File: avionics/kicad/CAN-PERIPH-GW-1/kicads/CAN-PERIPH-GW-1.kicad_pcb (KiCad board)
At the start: 2 copper layers, 49 x 25.5 mm, 32 parts, among them U1_1 MSPM0G3507, U2_1 SLB9670, U3_1 ISOW1044BDFMR, U4_1 ISOW1412

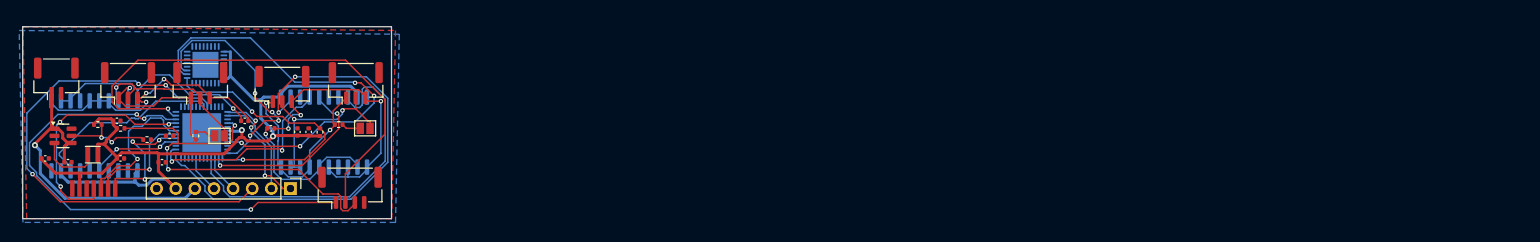
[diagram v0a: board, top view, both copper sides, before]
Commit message: just making everything shiny
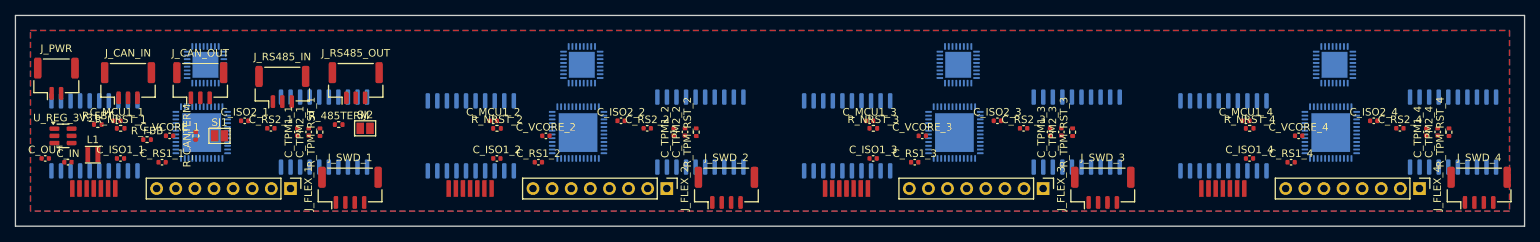
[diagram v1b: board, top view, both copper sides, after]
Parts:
- added C_ISO1_2: 100nF, Capacitor_SMD:C_0402_1005Metric, F.Cu at (194.0, 110.0)
- added C_ISO1_3: 100nF, Capacitor_SMD:C_0402_1005Metric, F.Cu at (244.0, 110.0)
- added C_ISO1_4: 100nF, Capacitor_SMD:C_0402_1005Metric, F.Cu at (294.0, 110.0)
- added C_ISO2_2: 1uF, Capacitor_SMD:C_0402_1005Metric, F.Cu at (210.5, 105.0)
- added C_ISO2_3: 1uF, Capacitor_SMD:C_0402_1005Metric, F.Cu at (260.5, 105.0)
- added C_ISO2_4: 1uF, Capacitor_SMD:C_0402_1005Metric, F.Cu at (310.5, 105.0)
- added C_MCU1_2: 100nF, Capacitor_SMD:C_0402_1005Metric, F.Cu at (193.5, 105.0)
- added C_MCU1_3: 100nF, Capacitor_SMD:C_0402_1005Metric, F.Cu at (243.5, 105.0)
- added C_MCU1_4: 100nF, Capacitor_SMD:C_0402_1005Metric, F.Cu at (293.5, 105.0)
- added C_RS1_2: 100nF, Capacitor_SMD:C_0402_1005Metric, F.Cu at (199.5, 110.5)
- added C_RS1_3: 100nF, Capacitor_SMD:C_0402_1005Metric, F.Cu at (249.5, 110.5)
- added C_RS1_4: 100nF, Capacitor_SMD:C_0402_1005Metric, F.Cu at (299.5, 110.5)
- added C_RS2_2: 100nF, Capacitor_SMD:C_0402_1005Metric, F.Cu at (213.9, 106.0)
- added C_RS2_3: 100nF, Capacitor_SMD:C_0402_1005Metric, F.Cu at (263.9, 106.0)
- added C_RS2_4: 100nF, Capacitor_SMD:C_0402_1005Metric, F.Cu at (313.9, 106.0)
- added C_TPM1_2: 100nF, Capacitor_SMD:C_0402_1005Metric, F.Cu at (217.5, 106.5)
- added C_TPM1_3: 100nF, Capacitor_SMD:C_0402_1005Metric, F.Cu at (267.5, 106.5)
- added C_TPM1_4: 100nF, Capacitor_SMD:C_0402_1005Metric, F.Cu at (317.5, 106.5)
- added C_TPM2_2: 1uF, Capacitor_SMD:C_0402_1005Metric, F.Cu at (219.0, 106.5)
- added C_TPM2_3: 1uF, Capacitor_SMD:C_0402_1005Metric, F.Cu at (269.0, 106.5)
- added C_TPM2_4: 1uF, Capacitor_SMD:C_0402_1005Metric, F.Cu at (319.0, 106.5)
- added C_VCORE_2: 1uF, Capacitor_SMD:C_0402_1005Metric, F.Cu at (200.5, 107.0)
- added C_VCORE_3: 1uF, Capacitor_SMD:C_0402_1005Metric, F.Cu at (250.5, 107.0)
- added C_VCORE_4: 1uF, Capacitor_SMD:C_0402_1005Metric, F.Cu at (300.5, 107.0)
- added J_ENC_2: AK7455 pigtail, Serenity-Custom:Pigtail_7W_DirectSolder, F.Cu at (190.4, 114.0)
- added J_ENC_3: AK7455 pigtail, Serenity-Custom:Pigtail_7W_DirectSolder, F.Cu at (240.4, 114.0)
- added J_ENC_4: AK7455 pigtail, Serenity-Custom:Pigtail_7W_DirectSolder, F.Cu at (290.4, 114.0)
- added J_FLEX_2: UART/TTL/PWM/BSHOT, Connector_PinHeader_2.54mm:PinHeader_1x08_P2.54mm_Vertical, F.Cu at (216.5, 114.0)
- added J_FLEX_3: UART/TTL/PWM/BSHOT, Connector_PinHeader_2.54mm:PinHeader_1x08_P2.54mm_Vertical, F.Cu at (266.5, 114.0)
- added J_FLEX_4: UART/TTL/PWM/BSHOT, Connector_PinHeader_2.54mm:PinHeader_1x08_P2.54mm_Vertical, F.Cu at (316.5, 114.0)
- added J_SWD_2: SWD, Connector_JST:JST_GH_BM04B-GHS-TBT_1x04-1MP_P1.25mm_Vertical, F.Cu at (224.5, 113.9)
- added J_SWD_3: SWD, Connector_JST:JST_GH_BM04B-GHS-TBT_1x04-1MP_P1.25mm_Vertical, F.Cu at (274.5, 113.9)
- added J_SWD_4: SWD, Connector_JST:JST_GH_BM04B-GHS-TBT_1x04-1MP_P1.25mm_Vertical, F.Cu at (324.5, 113.9)
- added R_NRST_2: 10k, Resistor_SMD:R_0402_1005Metric, F.Cu at (194.0, 106.0)
- added R_NRST_3: 10k, Resistor_SMD:R_0402_1005Metric, F.Cu at (244.0, 106.0)
- added R_NRST_4: 10k, Resistor_SMD:R_0402_1005Metric, F.Cu at (294.0, 106.0)
- added R_TPM_RST_2: 10k, Resistor_SMD:R_0402_1005Metric, F.Cu at (220.5, 106.5)
- added R_TPM_RST_3: 10k, Resistor_SMD:R_0402_1005Metric, F.Cu at (270.5, 106.5)
- added R_TPM_RST_4: 10k, Resistor_SMD:R_0402_1005Metric, F.Cu at (320.5, 106.5)
- added U1_2: MSPM0G3507, Package_DFN_QFN:QFN-48-1EP_7x7mm_P0.5mm_EP5.15x5.15mm, B.Cu at (204.8, 106.6)
- added U1_3: MSPM0G3507, Package_DFN_QFN:QFN-48-1EP_7x7mm_P0.5mm_EP5.15x5.15mm, B.Cu at (254.8, 106.6)
- added U1_4: MSPM0G3507, Package_DFN_QFN:QFN-48-1EP_7x7mm_P0.5mm_EP5.15x5.15mm, B.Cu at (304.8, 106.6)
- added U2_2: SLB9670, Package_DFN_QFN:QFN-32-1EP_5x5mm_P0.5mm_EP3.45x3.45mm, B.Cu at (205.2, 97.6)
- added U2_3: SLB9670, Package_DFN_QFN:QFN-32-1EP_5x5mm_P0.5mm_EP3.45x3.45mm, B.Cu at (255.2, 97.6)
- added U2_4: SLB9670, Package_DFN_QFN:QFN-32-1EP_5x5mm_P0.5mm_EP3.45x3.45mm, B.Cu at (305.2, 97.6)
- added U3_2: ISOW1044BDFMR, Package_SO:SOIC-20W_7.5x12.8mm_P1.27mm, B.Cu at (190.5, 107.0)
- added U3_3: ISOW1044BDFMR, Package_SO:SOIC-20W_7.5x12.8mm_P1.27mm, B.Cu at (240.5, 107.0)
- added U3_4: ISOW1044BDFMR, Package_SO:SOIC-20W_7.5x12.8mm_P1.27mm, B.Cu at (290.5, 107.0)
- added U4_2: ISOW1412, Package_SO:SOIC-20W_7.5x12.8mm_P1.27mm, B.Cu at (221.0, 106.5)
- added U4_3: ISOW1412, Package_SO:SOIC-20W_7.5x12.8mm_P1.27mm, B.Cu at (271.0, 106.5)
- added U4_4: ISOW1412, Package_SO:SOIC-20W_7.5x12.8mm_P1.27mm, B.Cu at (321.0, 106.5)
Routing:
- net +3V3: track 112.6 -> 0.00 mm, vias 2 -> 0
- net MCU_SWDIO_1: track 68.4 -> 0.00 mm, vias 3 -> 0
- net FLEX_TTL_GPIO_1: track 67.3 -> 0.00 mm, vias 3 -> 0
- net MCU_SWCLK_1: track 67.2 -> 0.00 mm, vias 1 -> 0
- net RS485_TX_1: track 64.0 -> 0.00 mm, vias 2 -> 0
- net TPM_PIRQ_1: track 56.8 -> 0.00 mm, vias 4 -> 0
- net MCU_NRST_1: track 52.5 -> 0.00 mm, vias 3 -> 0
- net RS485_FLT_N_1: track 45.7 -> 0.00 mm
- net +5V: track 40.9 -> 0.00 mm, vias 1 -> 0
- net ISO_GND_485: track 38.0 -> 0.00 mm, vias 3 -> 0
- net TPM_RESET_N_1: track 37.5 -> 0.00 mm, vias 2 -> 0
- net ISO_GND_CAN: track 35.1 -> 0.00 mm, vias 3 -> 0
- net TPM_SPI_SCK_1: track 32.2 -> 0.00 mm, vias 4 -> 0
- net ENC_SPI_MOSI_1: track 32.1 -> 0.00 mm, vias 3 -> 0
- net ISO_5V_CAN_1: track 30.6 -> 0.00 mm, vias 1 -> 0
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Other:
- board size 49 x 25.5 mm -> 200.5 x 28 mm
- board text added: "TPM-Secured CAN-FD/RS-485 Gateway For the PocketBeagle2 fleet CC BY 4.0 — July 2026 Steve Griffing PE(CSE), CISSP-ISSEP, CPP Griffing Technology LLC github.com/Stab-Rabbit-Coding"

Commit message: who's flying this thing
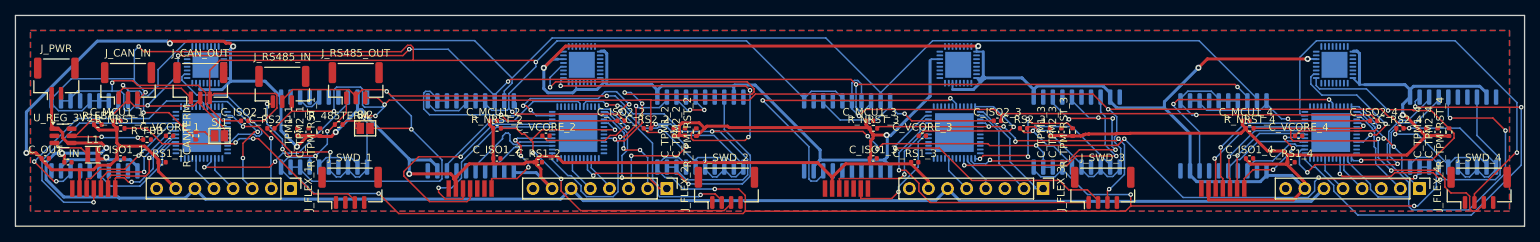
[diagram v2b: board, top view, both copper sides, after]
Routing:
- net +3V3: track 0.00 -> 632.3 mm, vias 0 -> 13
- net ISO_GND_CAN: track 0.00 -> 307.9 mm, vias 0 -> 6
- net ISO_GND_485: track 0.00 -> 256.9 mm, vias 0 -> 8
- net RS485_A: track 0.00 -> 232.5 mm, vias 0 -> 8
- net RS485_B: track 0.00 -> 231.8 mm, vias 0 -> 10
- net +5V: track 0.00 -> 200.8 mm, vias 0 -> 2
- net CAN_H: track 0.00 -> 197.3 mm, vias 0 -> 2
- net CAN_L: track 0.00 -> 184.1 mm, vias 0 -> 7
- net RS485_DE_4: track 0.00 -> 61.2 mm, vias 0 -> 2
- net TPM_SPI_CS_2: track 0.00 -> 61.0 mm, vias 0 -> 4
- net RS485_TX_4: track 0.00 -> 59.1 mm, vias 0 -> 2
- net MCU_SWCLK_4: track 0.00 -> 57.1 mm, vias 0 -> 1
- net MCU_NRST_2: track 0.00 -> 51.0 mm, vias 0 -> 3
- net MCU_NRST_4: track 0.00 -> 50.6 mm, vias 0 -> 3
- net MCU_NRST_3: track 0.00 -> 44.5 mm, vias 0 -> 5
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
